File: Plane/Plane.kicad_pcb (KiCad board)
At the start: 2 copper layers, 58 x 71.5 mm, 28 parts, among them J1 SPI Bus 17, J2 SPI Bus 5, M1 Aileron_Left, M2 Aileron_Right, M3 Elevator, M4 Rudder, M5 Speed Controller, M6 Unassigned, M7 Unassigned, U1 Left Ranging, U10 I2C, U11 PitotPX4, U2 Right Ranging, U3 PX4TelemRadio, U4 TBD Ranging, U5 IMU, U6 Baro, U7 MissionComputerSerial, U8 TPS2117DRLR

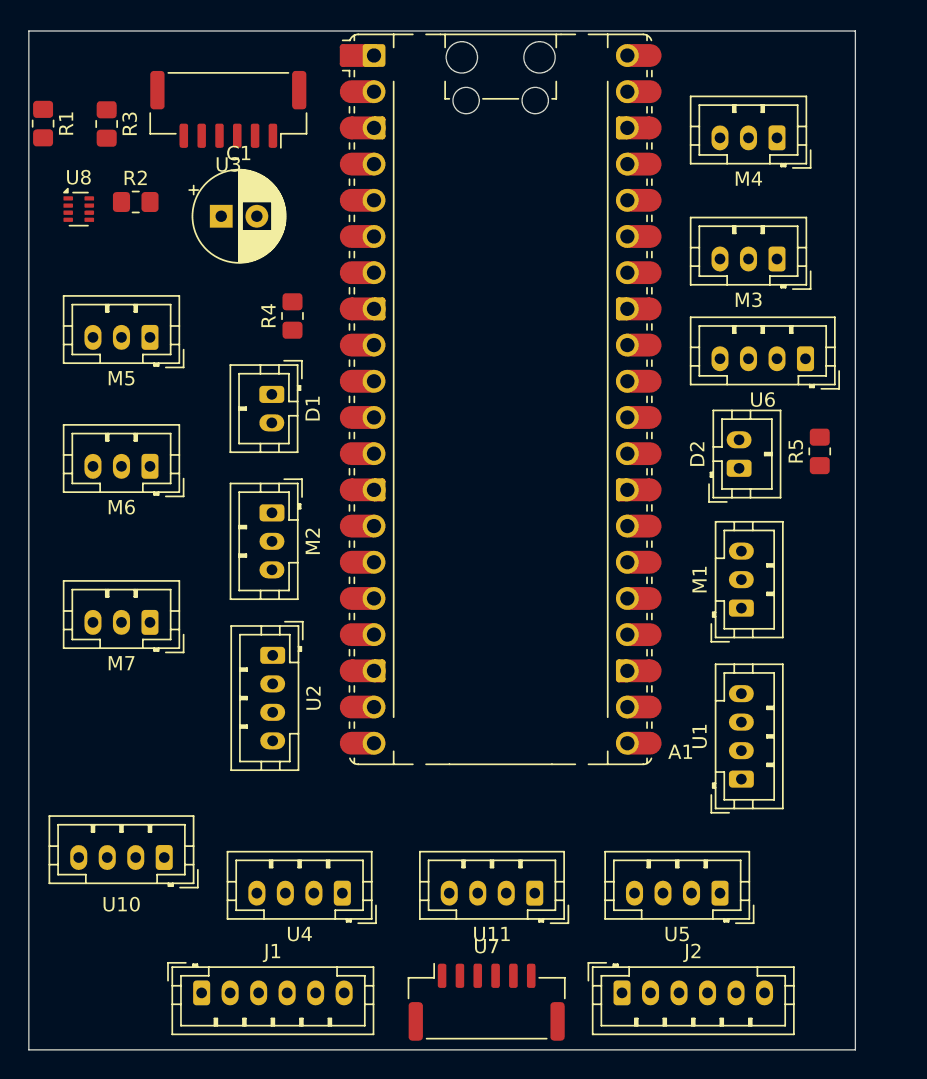
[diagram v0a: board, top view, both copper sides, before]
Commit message: finish routing
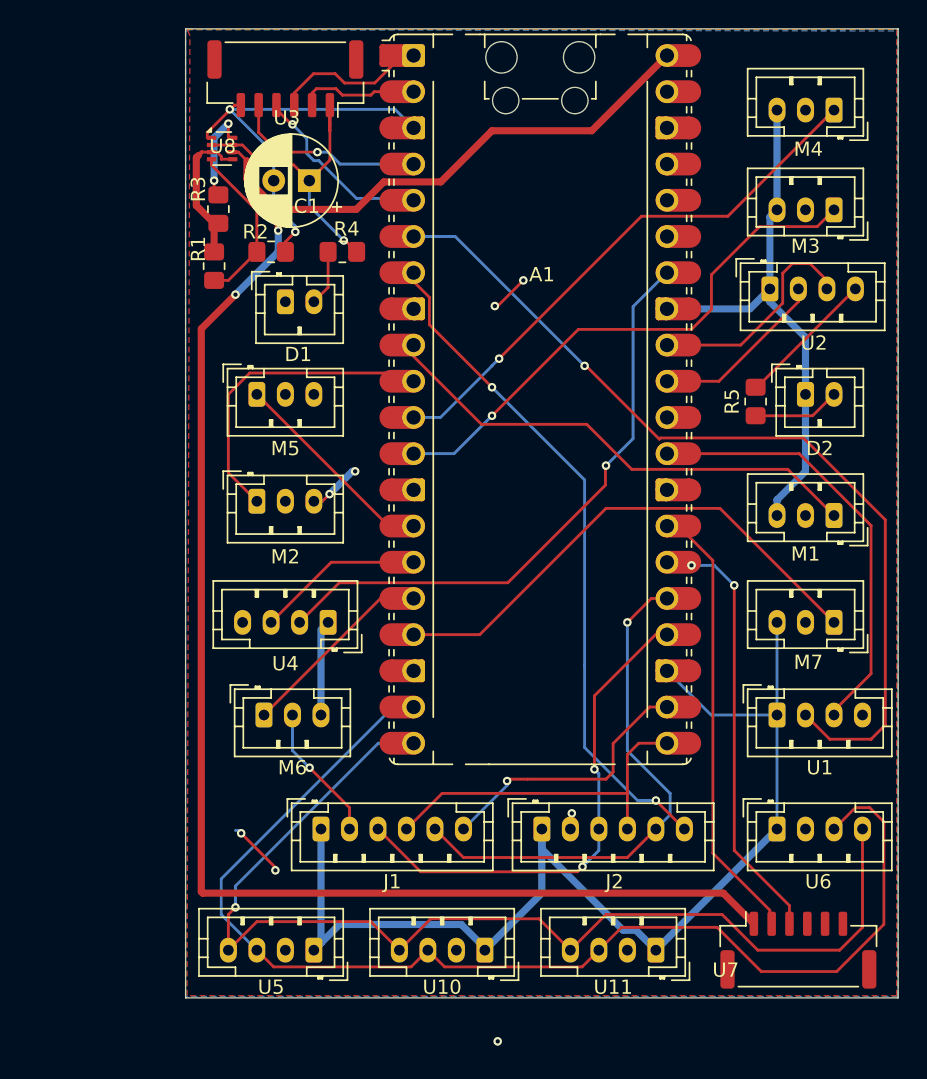
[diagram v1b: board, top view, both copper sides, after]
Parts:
- moved M7 48.0 mm to (233.0, 121.0)
- moved U2 43.3 mm to (228.5, 97.6), turned to 0 degrees
- moved U6 33.1 mm to (229.0, 135.5), turned to 0 degrees
- moved U5 28.8 mm to (196.5, 144.0)
- moved U10 23.4 mm to (208.5, 144.0)
- moved U7 22.2 mm to (230.5, 144.0)
- moved M6 19.2 mm to (193.0, 127.5), turned to 0 degrees
- moved U4 19.0 mm to (197.5, 121.0)
- moved R1 15.6 mm to (189.5, 96.0)
- moved J1 14.2 mm to (197.0, 135.5)
- moved J2 12.8 mm to (212.5, 135.5)
- moved U8 10.9 mm to (190.1, 87.8)
- moved R2 10.1 mm to (193.5, 95.0)
- moved R3 9.86 mm to (189.8, 92.0)
- moved U11 9.39 mm to (220.5, 144.0)
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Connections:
- A1 pad 2: /radio_rx_mcu_rx -> /radio_tx_mcu_rx
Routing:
- net GND: track 0.00 -> 158.3 mm, vias 0 -> 4
- net /VUSB: track 0.00 -> 127.6 mm, vias 0 -> 2
- net /i2c_sda: track 0.00 -> 85.5 mm
- net /i2c_scl: track 0.00 -> 79.0 mm, vias 0 -> 1
- net /range_1_trig: track 0.00 -> 62.8 mm, vias 0 -> 1
- net /spi_cs_5: track 0.00 -> 48.1 mm, vias 0 -> 2
- net +5V: track 0.00 -> 42.9 mm, vias 0 -> 3
- net /range_3_trig: track 0.00 -> 42.1 mm, vias 0 -> 1
- net /rudder: track 0.00 -> 38.4 mm, vias 0 -> 1
- net /elevator: track 0.00 -> 38.1 mm, vias 0 -> 1
- net /spi_mosi: track 0.00 -> 37.6 mm, vias 0 -> 1
- net /m7: track 0.00 -> 37.3 mm
- net /spi_clock: track 0.00 -> 36.0 mm, vias 0 -> 2
- net /aileron_left: track 0.00 -> 35.3 mm
- net /mission_tx_mcu_rx: track 0.00 -> 30.6 mm
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- added copper zone on B.Cu, net +5V
- added copper zone on F.Cu, net GND
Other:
- board size 58 x 71.5 mm -> 50 x 68 mm
